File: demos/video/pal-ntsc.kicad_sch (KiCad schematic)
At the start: 36 parts, among them U10 BT812, X2 30MHz

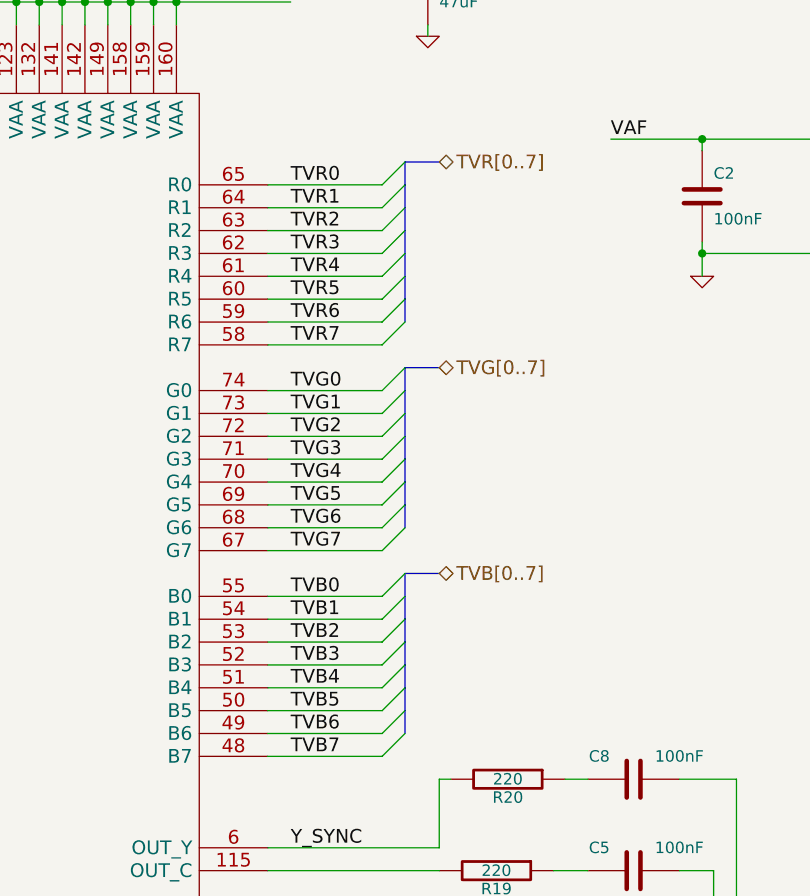
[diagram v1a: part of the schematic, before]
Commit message: Update demos.
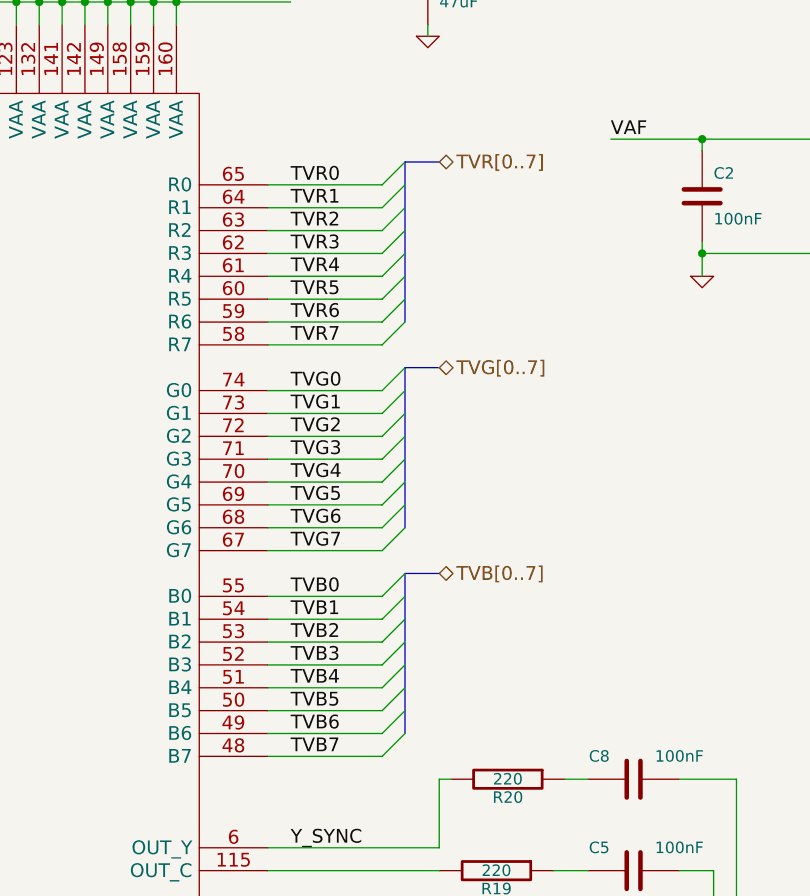
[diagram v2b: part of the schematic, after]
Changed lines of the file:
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@@
-(kicad_sch (version 20210126) (generator eeschema)
+(kicad_sch (version 20210406) (generator eeschema)
   (paper "A3")
   (title_block
@@
     (stroke (width 0) (type solid) (color 0 0 0 0))
   )
-  (bus (pts (xy 270.51 78.74) (xy 270.51 81.28))
-    (stroke (width 0) (type solid) (color 0 0 0 0))
-  )
-  (bus (pts (xy 270.51 81.28) (xy 270.51 83.82))
-    (stroke (width 0) (type solid) (color 0 0 0 0))
-  )
-  (bus (pts (xy 270.51 83.82) (xy 270.51 86.36))
-    (stroke (width 0) (type solid) (color 0 0 0 0))
-  )
-  (bus (pts (xy 270.51 86.36) (xy 270.51 88.9))
-    (stroke (width 0) (type solid) (color 0 0 0 0))
-  )
-  (bus (pts (xy 270.51 88.9) (xy 270.51 91.44))
-    (stroke (width 0) (type solid) (color 0 0 0 0))
-  )
-  (bus (pts (xy 270.51 91.44) (xy 270.51 93.98))
-    (stroke (width 0) (type solid) (color 0 0 0 0))
-  )
-  (bus (pts (xy 270.51 93.98) (xy 270.51 96.52))
-    (stroke (width 0) (type solid) (color 0 0 0 0))
-  )
-  (bus (pts (xy 270.51 101.6) (xy 270.51 104.14))
-    (stroke (width 0) (type solid) (color 0 0 0 0))
-  )
-  (bus (pts (xy 270.51 104.14) (xy 270.51 106.68))
-    (stroke (width 0) (type solid) (color 0 0 0 0))
-  )
-  (bus (pts (xy 270.51 106.68) (xy 270.51 109.22))
-    (stroke (width 0) (type solid) (color 0 0 0 0))
-  )
-  (bus (pts (xy 270.51 109.22) (xy 270.51 111.76))
-    (stroke (width 0) (type solid) (color 0 0 0 0))
-  )
-  (bus (pts (xy 270.51 111.76) (xy 270.51 114.3))
-    (stroke (width 0) (type solid) (color 0 0 0 0))
-  )
-  (bus (pts (xy 270.51 114.3) (xy 270.51 116.84))
-    (stroke (width 0) (type solid) (color 0 0 0 0))
-  )
-  (bus (pts (xy 270.51 116.84) (xy 270.51 119.38))
-    (stroke (width 0) (type solid) (color 0 0 0 0))
-  )
-  (bus (pts (xy 270.51 124.46) (xy 270.51 127))
-    (stroke (width 0) (type solid) (color 0 0 0 0))
-  )
-  (bus (pts (xy 270.51 127) (xy 270.51 129.54))
-    (stroke (width 0) (type solid) (color 0 0 0 0))
-  )
-  (bus (pts (xy 270.51 129.54) (xy 270.51 132.08))
-    (stroke (width 0) (type solid) (color 0 0 0 0))
-  )
-  (bus (pts (xy 270.51 132.08) (xy 270.51 134.62))
-    (stroke (width 0) (type solid) (color 0 0 0 0))
-  )
-  (bus (pts (xy 270.51 134.62) (xy 270.51 137.16))
-    (stroke (width 0) (type solid) (color 0 0 0 0))
-  )
-  (bus (pts (xy 270.51 137.16) (xy 270.51 139.7))
-    (stroke (width 0) (type solid) (color 0 0 0 0))
-  )
-  (bus (pts (xy 270.51 139.7) (xy 270.51 142.24))
-    (stroke (width 0) (type solid) (color 0 0 0 0))
-  )
+  (bus (pts (xy 270.51 78.74) (xy 270.51 96.52))
+    (stroke (width 0) (type solid) (color 0 0 0 0))
+  )
+  (bus (pts (xy 270.51 101.6) (xy 270.51 119.38))
+    (stroke (width 0) (type solid) (color 0 0 0 0))
+  )
+  (bus (pts (xy 270.51 124.46) (xy 270.51 142.24))
+    (stroke (width 0) (type solid) (color 0 0 0 0))
+  )

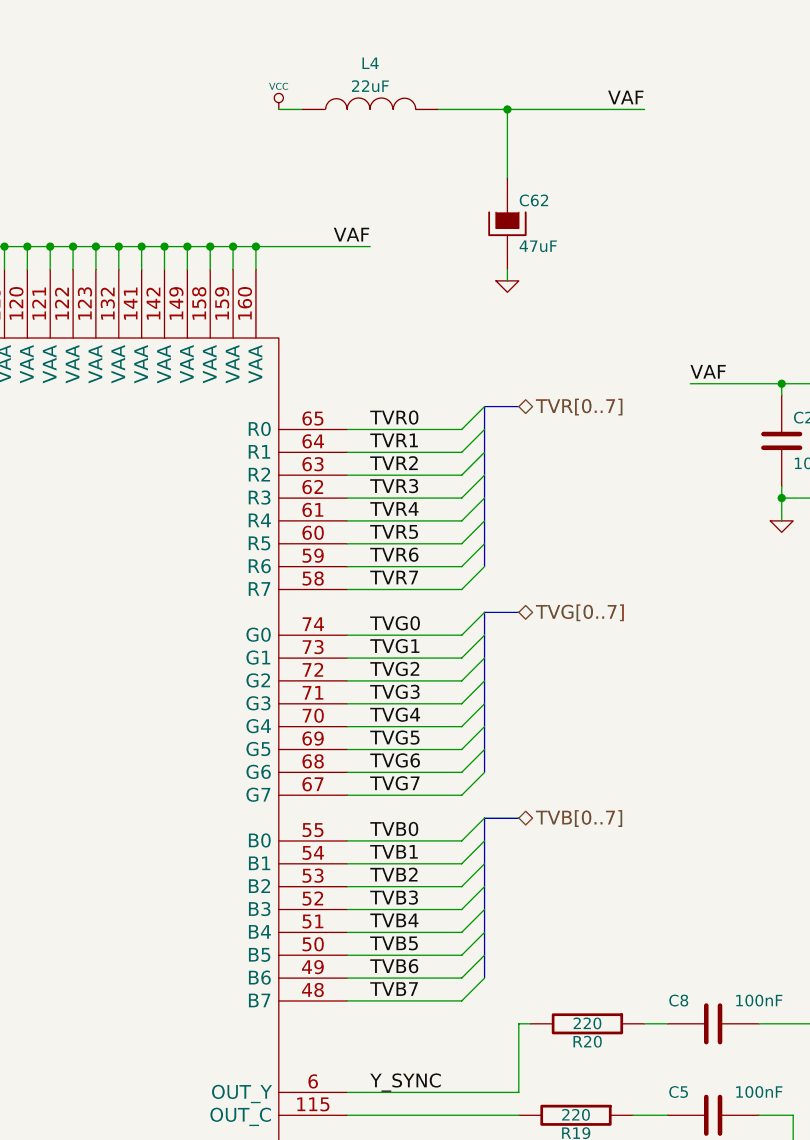
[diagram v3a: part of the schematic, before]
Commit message: Demos update.
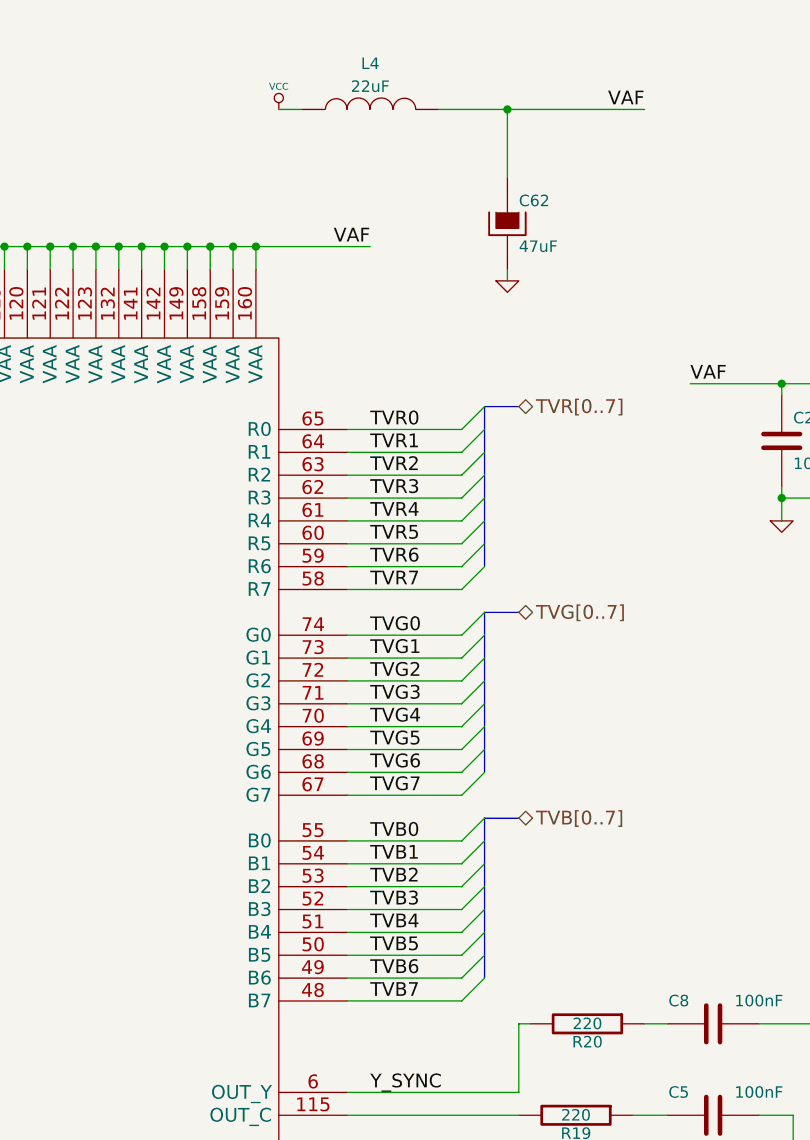
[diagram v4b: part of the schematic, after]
